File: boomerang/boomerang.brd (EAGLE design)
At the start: 54.1 x 59.6 mm, 11 parts, among them IC1 WS2811-SOP8, X3 87438-06

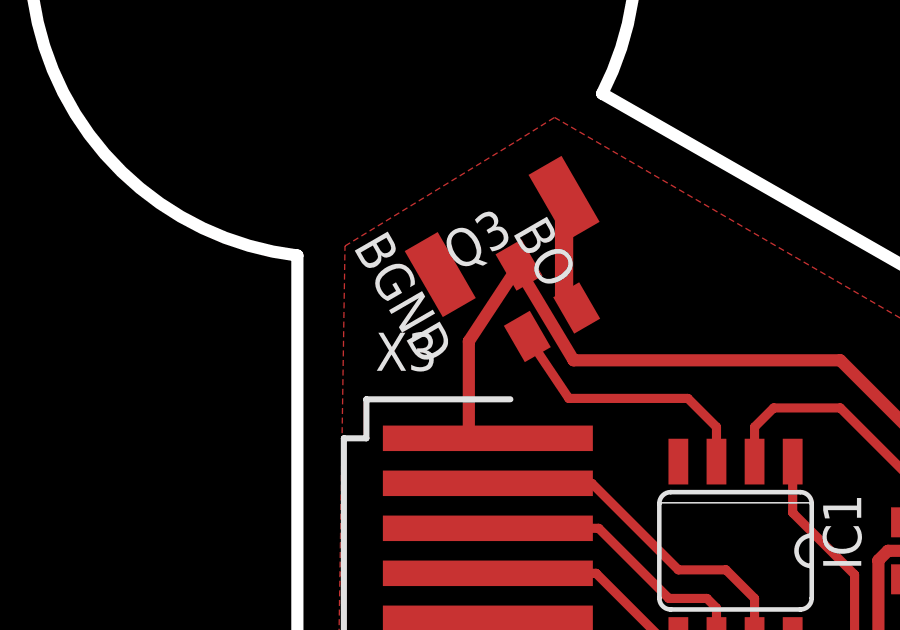
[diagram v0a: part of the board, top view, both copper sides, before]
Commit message: OCD for everyone
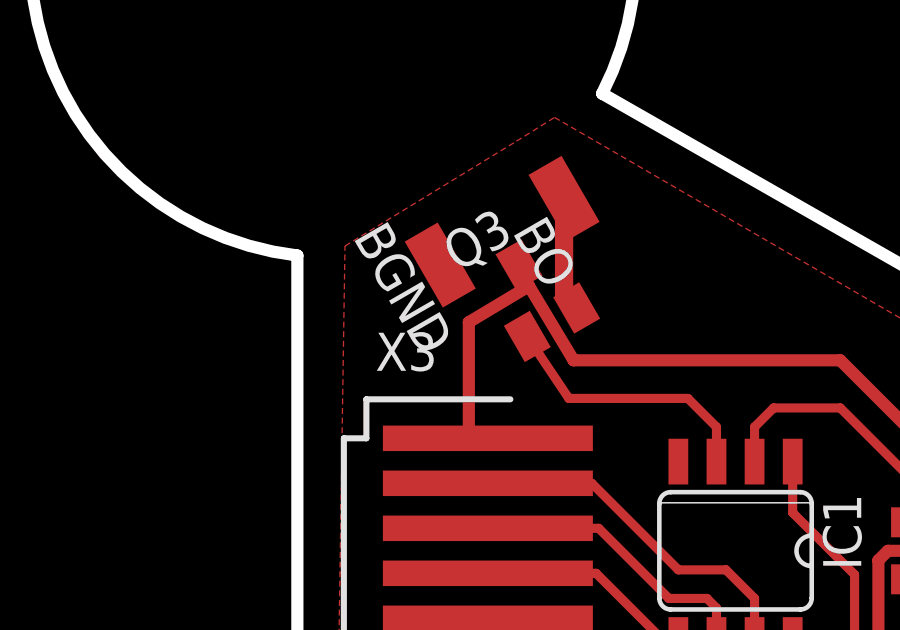
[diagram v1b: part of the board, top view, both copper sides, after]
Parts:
- moved BGND 0.32 mm to (-7.94, 9.53)
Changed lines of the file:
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@@
 <element name="RGND" library="wirepad" package="SMD1,27-2,54" value="" x="-4.445" y="-11.43" rot="R150"/>
 <element name="GGND" library="wirepad" package="SMD1,27-2,54" value="" x="11.115" y="2" rot="R270"/>
-<element name="BGND" library="wirepad" package="SMD1,27-2,54" value="" x="-7.9375" y="9.2075" rot="R30"/>
+<element name="BGND" library="wirepad" package="SMD1,27-2,54" value="" x="-7.9375" y="9.525" rot="R30"/>
 <element name="Q1" library="adafruit" package="SOT23" value="" x="-5.08" y="-8.5725" rot="R150"/>
 <element name="Q2" library="adafruit" package="SOT23" value="" x="8.89" y="0" rot="R270"/>
@@
 <contactref element="X3" pad="6"/>
 <wire x1="-6.35" y1="-2.25" x2="-6.35" y2="-3.75" width="0.4064" layer="1"/>
-<polygon width="0.6096" layer="1">
+<polygon width="0.6096" layer="1" isolate="0.4064" orphans="yes">
 <vertex x="-4.1275" y="14.44625"/>
 <vertex x="13.6525" y="4.1275"/>
@@
 <contactref element="Q3" pad="3"/>
 <contactref element="X3" pad="1"/>
-<wire x1="-5.3125" y1="9.525125" x2="-6.985" y2="6.985" width="0.4064" layer="1"/>
-<wire x1="-6.985" y1="6.985" x2="-6.985" y2="3.81" width="0.4064" layer="1"/>
+<wire x1="-6.985" y1="7.62" x2="-6.985" y2="3.81" width="0.4064" layer="1"/>
 <wire x1="-6.985" y1="3.81" x2="-3.87" y2="3.81" width="0.4064" layer="1"/>
 <wire x1="-3.87" y1="3.81" x2="-6.35" y2="3.75" width="0.4064" layer="1"/>
@@
 <wire x1="8.89" y1="0" x2="6.985" y2="0" width="0.4064" layer="1"/>
 <wire x1="6.985" y1="0" x2="6.6675" y2="-0.3175" width="0.4064" layer="1"/>
-<wire x1="-5.3975" y1="9.525" x2="-3.4925" y2="6.35" width="0.4064" layer="1"/>
+<wire x1="-5.3975" y1="9.525" x2="-4.977278125" y2="8.82463125" width="0.4064" layer="1"/>
+<wire x1="-4.977278125" y1="8.82463125" x2="-3.4925" y2="6.35" width="0.4064" layer="1"/>
 <wire x1="-3.4925" y1="6.35" x2="5.3975" y2="6.35" width="0.4064" layer="1"/>
 <wire x1="5.3975" y1="6.35" x2="8.89" y2="2.8575" width="0.4064" layer="1"/>
@@
 <wire x1="-5.08" y1="-8.73125" x2="-1.905" y2="-10.63625" width="0.4064" layer="1"/>
 <wire x1="-1.905" y1="-10.63625" x2="-1.27" y2="-10.795" width="0.4064" layer="1"/>
+<wire x1="-6.985" y1="7.62" x2="-4.977278125" y2="8.82463125" width="0.4064" layer="1"/>
 <wire x1="-5.3975" y1="9.525" x2="-5.3125" y2="9.525125" width="0" layer="19" extent="1-1"/>
 </signal>
